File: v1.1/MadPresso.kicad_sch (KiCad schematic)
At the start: 42 parts, among them J1 Conn_01x07, J2 Conn_01x03, J3 Conn_01x02, J4 Conn_01x04, Q1 BC847, Q2 BSS84, U1 LTV-356T, U2 ADC101C021CIMK, U3 WeMos_D1_mini

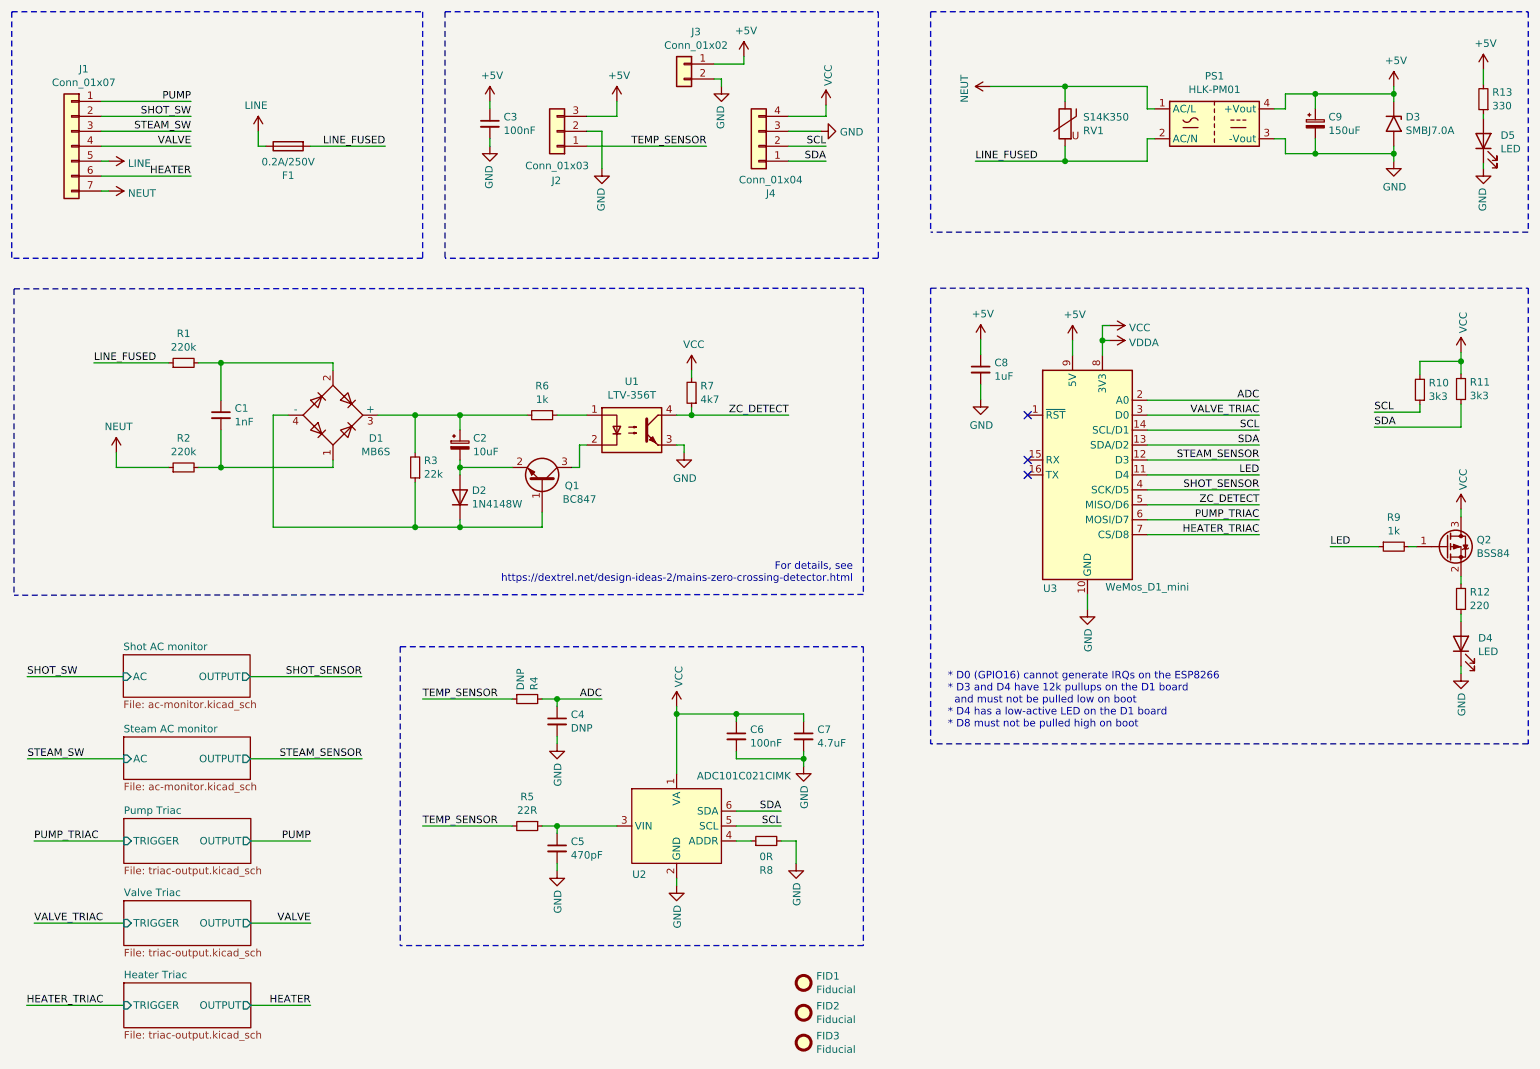
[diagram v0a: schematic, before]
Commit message: more routing
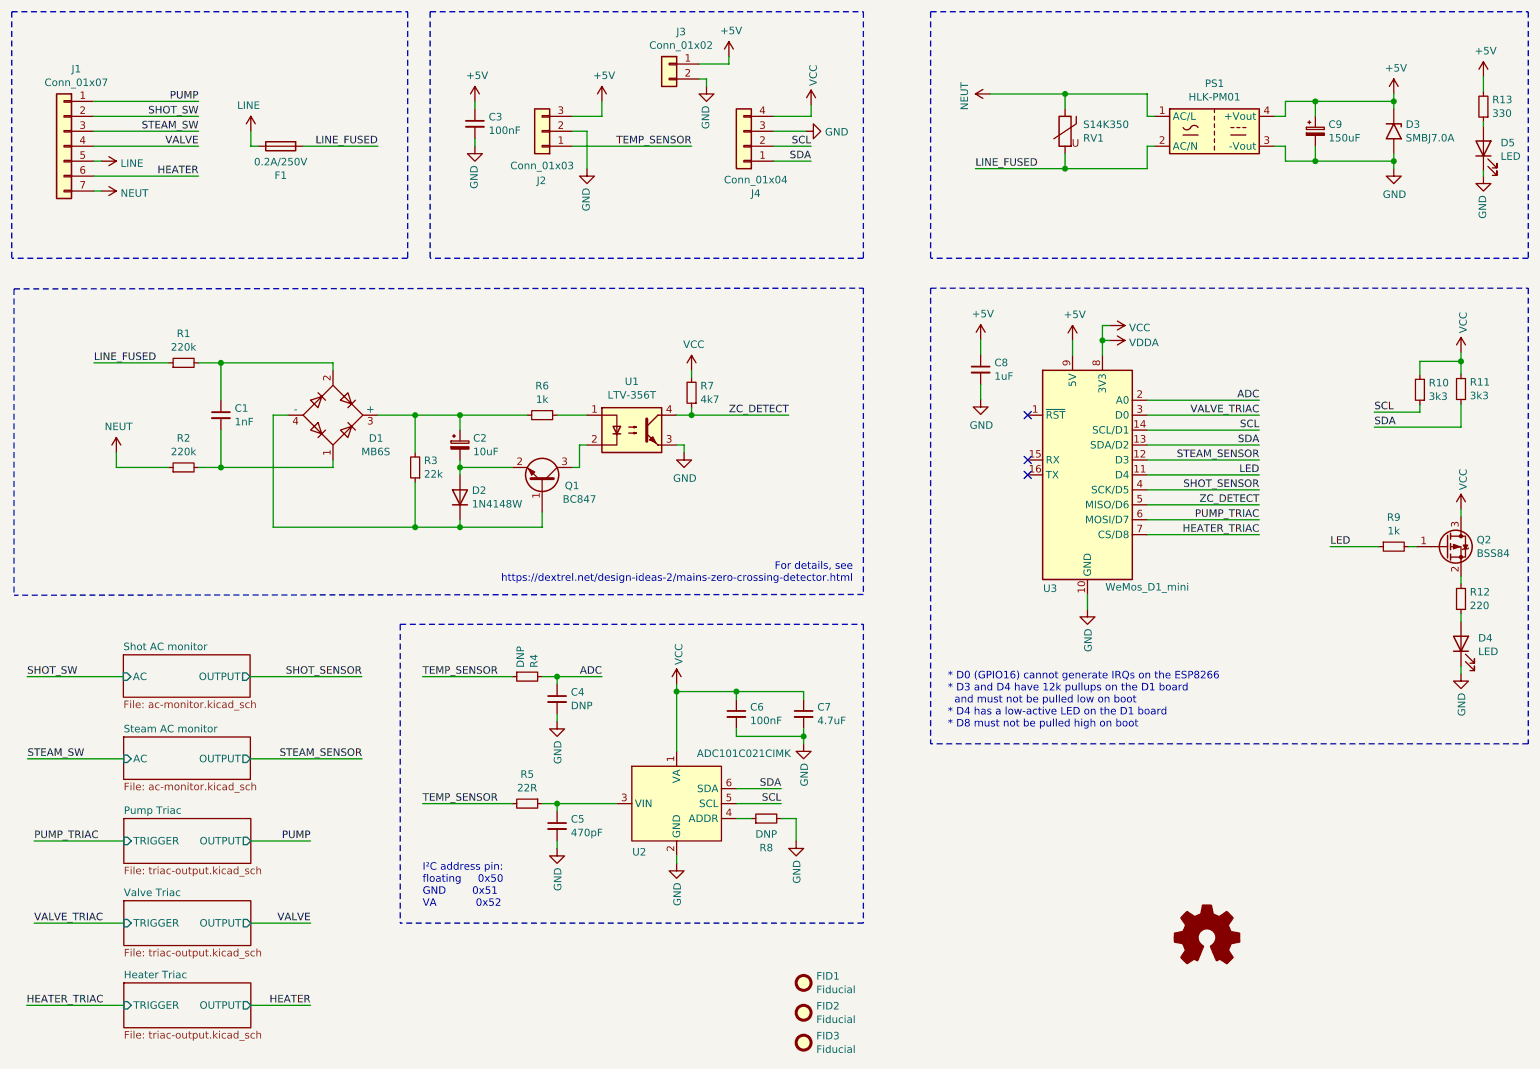
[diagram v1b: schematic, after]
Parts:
- R8: value 0R -> DNP
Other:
- note added: "I²C address pin: floating 0x50 GND 0x51 VA 0x52"
- title: (none) -> MadPresso controller
- moved on the sheet: C3, C4, C5, C6, C7, C9, D3, D5, F1, J1, J2, J3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

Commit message: some more documentation
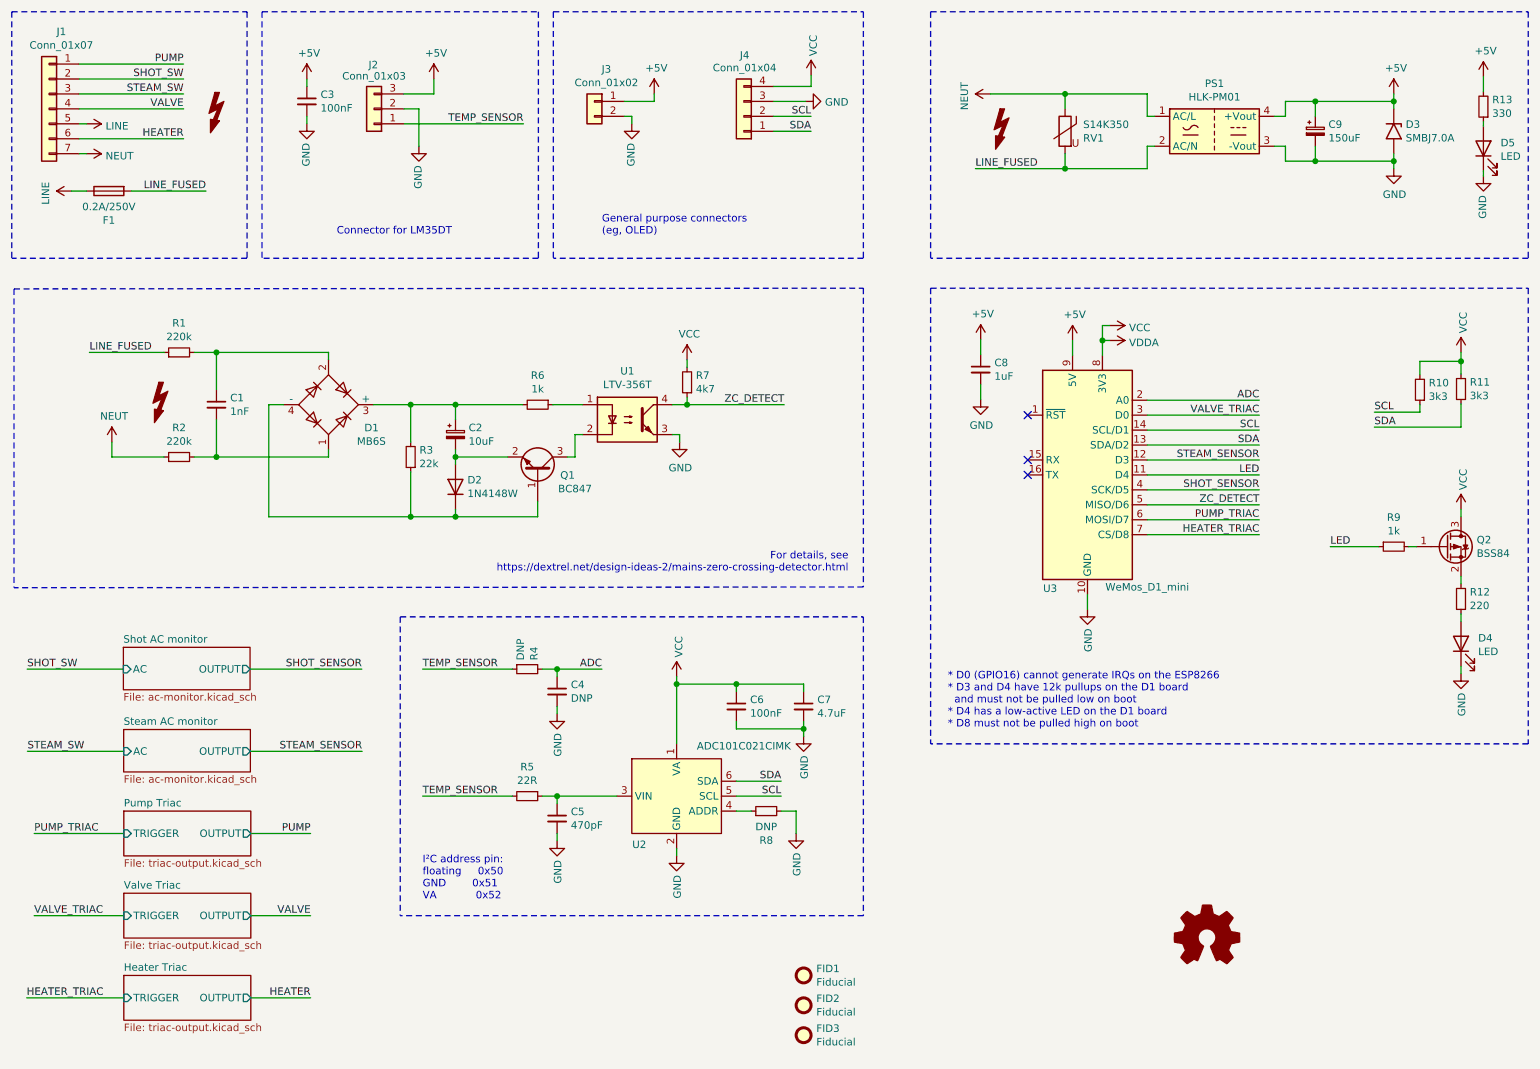
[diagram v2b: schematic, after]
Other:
- note added: "Connector for LM35DT"
- note added: "General purpose connectors (eg, OLED)"
- moved on the sheet: C1, C2, C3, C4, C5, C6, C7, D1, D2, F1, FID1, FID2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

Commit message: v1.1a
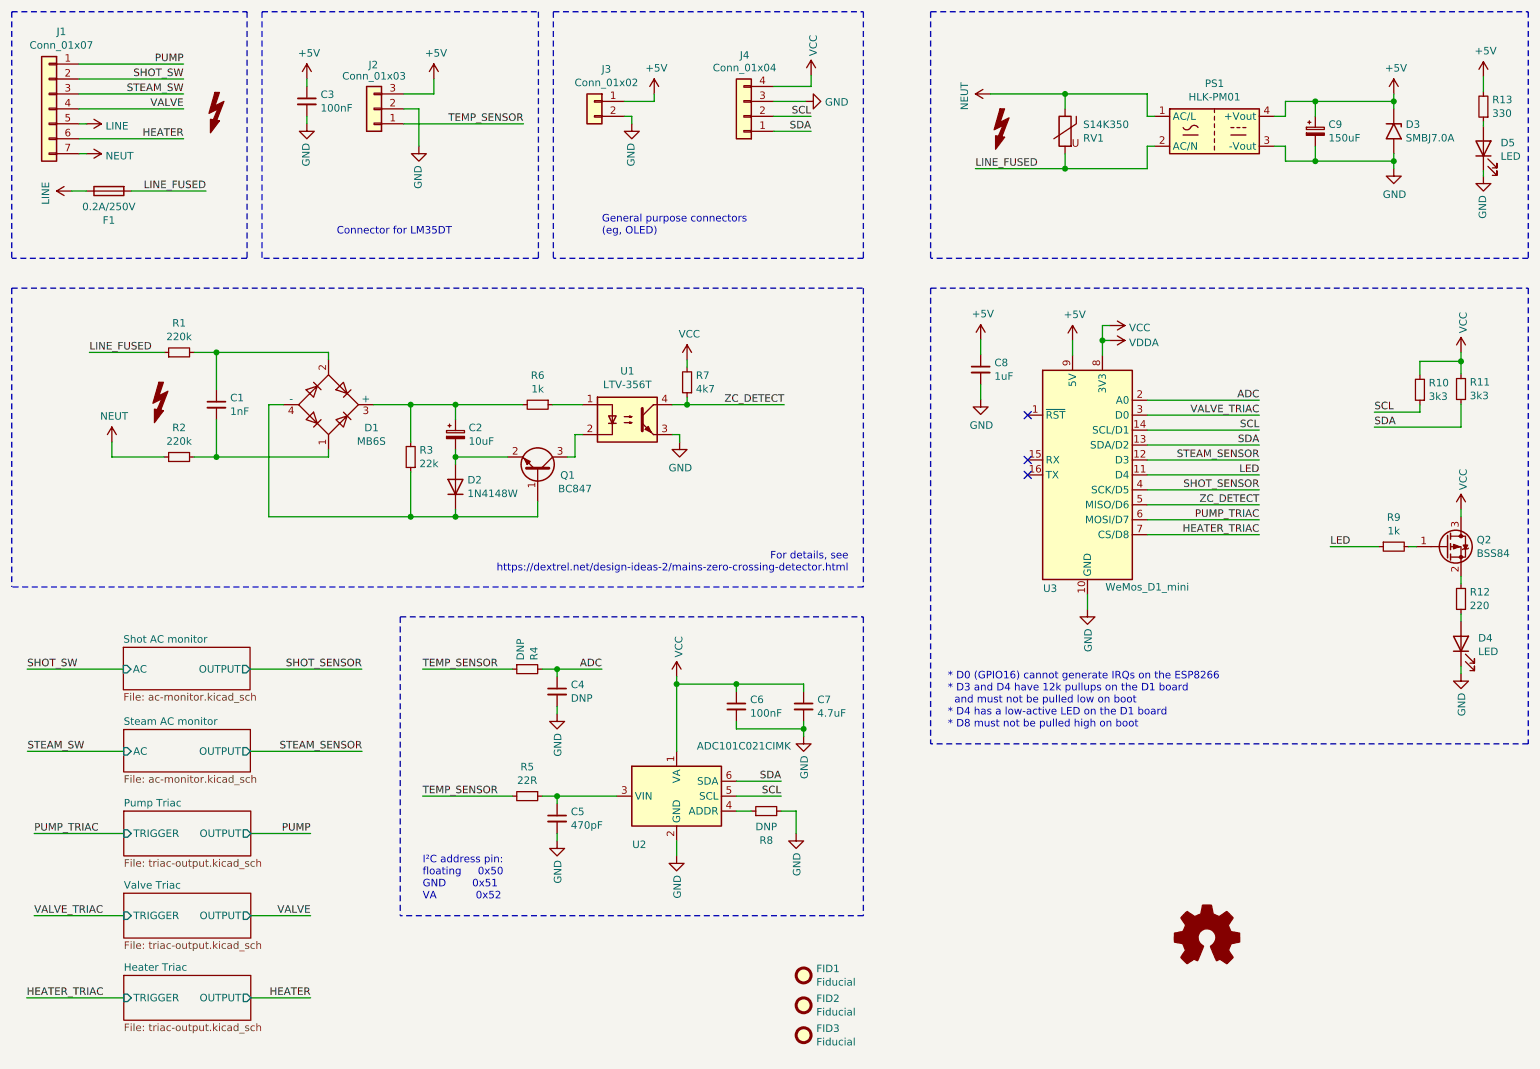
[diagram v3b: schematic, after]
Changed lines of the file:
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@@
   (junction (at 255.27 41.91) (diameter 1.016) (color 0 0 0 0))
   (junction (at 266.7 75.946) (diameter 1.016) (color 0 0 0 0))
-  (no_connect (at 193.04 95.25))
   (no_connect (at 193.04 85.09))
   (no_connect (at 193.04 92.71))
+  (no_connect (at 193.04 95.25))
   (wire (pts (xy 22.86 184.15) (xy 39.37 184.15))
     (stroke (width 0) (type solid) (color 0 0 0 0))
@@
     (stroke (width 0) (type solid) (color 0 0 0 0))
   )
-  (wire (pts (xy 133.35 130.81) (xy 133.35 140.97))
+  (wire (pts (xy 133.35 130.81) (xy 133.35 142.24))
     (stroke (width 0) (type solid) (color 0 0 0 0))
   )
@@
     (stroke (width 0) (type solid) (color 0 0 0 0))
   )
-  (wire (pts (xy 133.35 158.75) (xy 133.35 160.02))
+  (wire (pts (xy 133.35 157.48) (xy 133.35 160.02))
     (stroke (width 0) (type solid) (color 0 0 0 0))
   )
@@
     (stroke (width 0) (type dash) (color 0 0 0 0))
   )
-  (polyline (pts (xy 20.701 63.627) (xy 20.701 114.427))
-    (stroke (width 0) (type dash) (color 0 0 0 0))
-  )
-  (polyline (pts (xy 20.701 63.627) (xy 165.1 63.5))
+  (polyline (pts (xy 20.32 63.5) (xy 20.32 114.3))
+    (stroke (width 0) (type dash) (color 0 0 0 0))
+  )
+  (polyline (pts (xy 20.32 63.5) (xy 165.1 63.5))
     (stroke (width 0) (type dash) (color 0 0 0 0))
   )
@@
     (stroke (width 0) (type dash) (color 0 0 0 0))
   )
-  (polyline (pts (xy 165.1 114.3) (xy 20.701 114.427))
-    (stroke (width 0) (type dash) (color 0 0 0 0))
-  )
+  (polyline (pts (xy 165.1 114.3) (xy 20.32 114.3))
+    (stroke (width 0) (type dash) (color 0 0 0 0))
+  )
